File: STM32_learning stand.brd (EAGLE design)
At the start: 100 x 90 mm, 131 parts, among them J1 Power in, J10 RS-485_1, J11 RS-485_2, J12 FD CAN 1, J13 FD CAN 2, J15 Motor, J2 ST-link, J3 Encoder, J4 BMS_interface, J5 S6B-PH-K, J6 Current_1, J7 Current_2, J8 I2C, U1 TPS7A19, U10 THDV1450, U11 TCAN1042HGV, U12 DRV8701, U2 SGM2019, U3 STM32G431CBT, U4 REF3330, U5 REF3318, U6 ACS711KEXLT-15AB-T, U7 INA240A1, U8 24LC64T-I/SN, U9 CP2102N-A01-GQFN20, X1 CSTNE

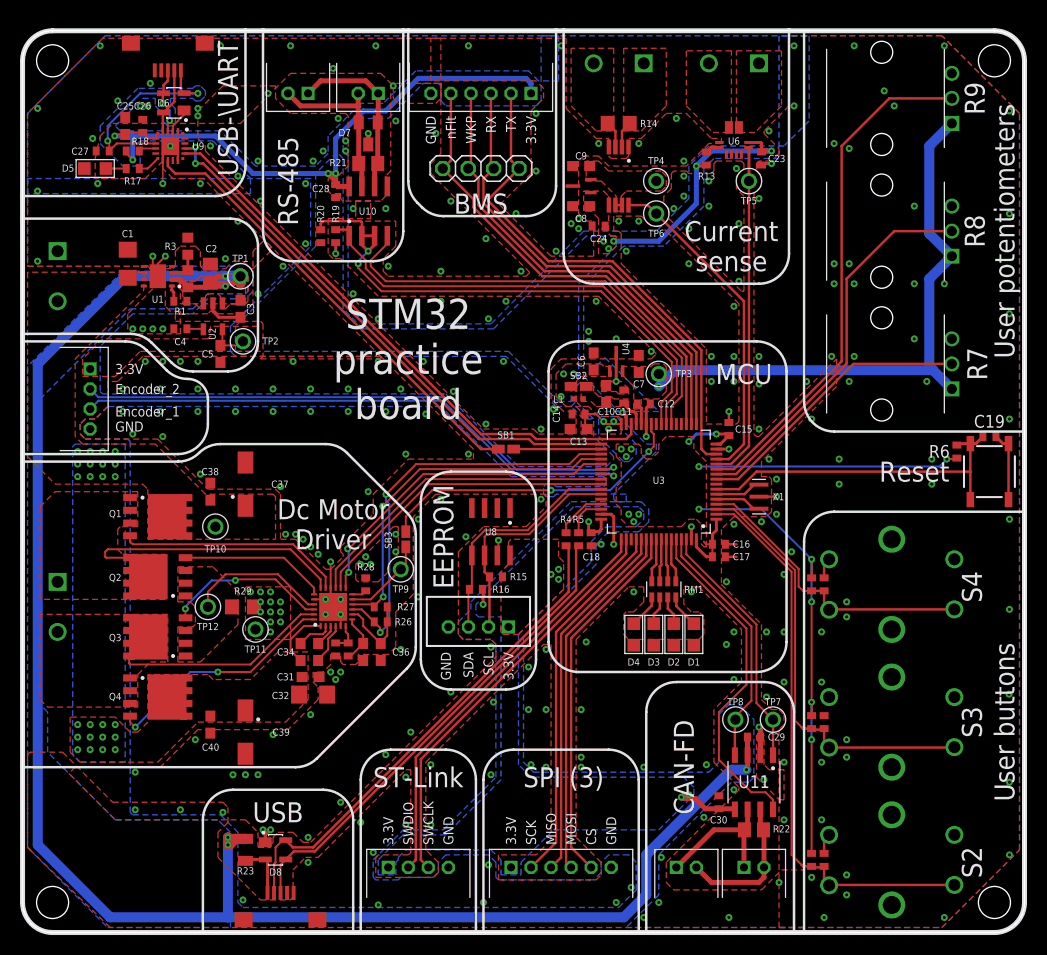
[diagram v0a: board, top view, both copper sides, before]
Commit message: small update
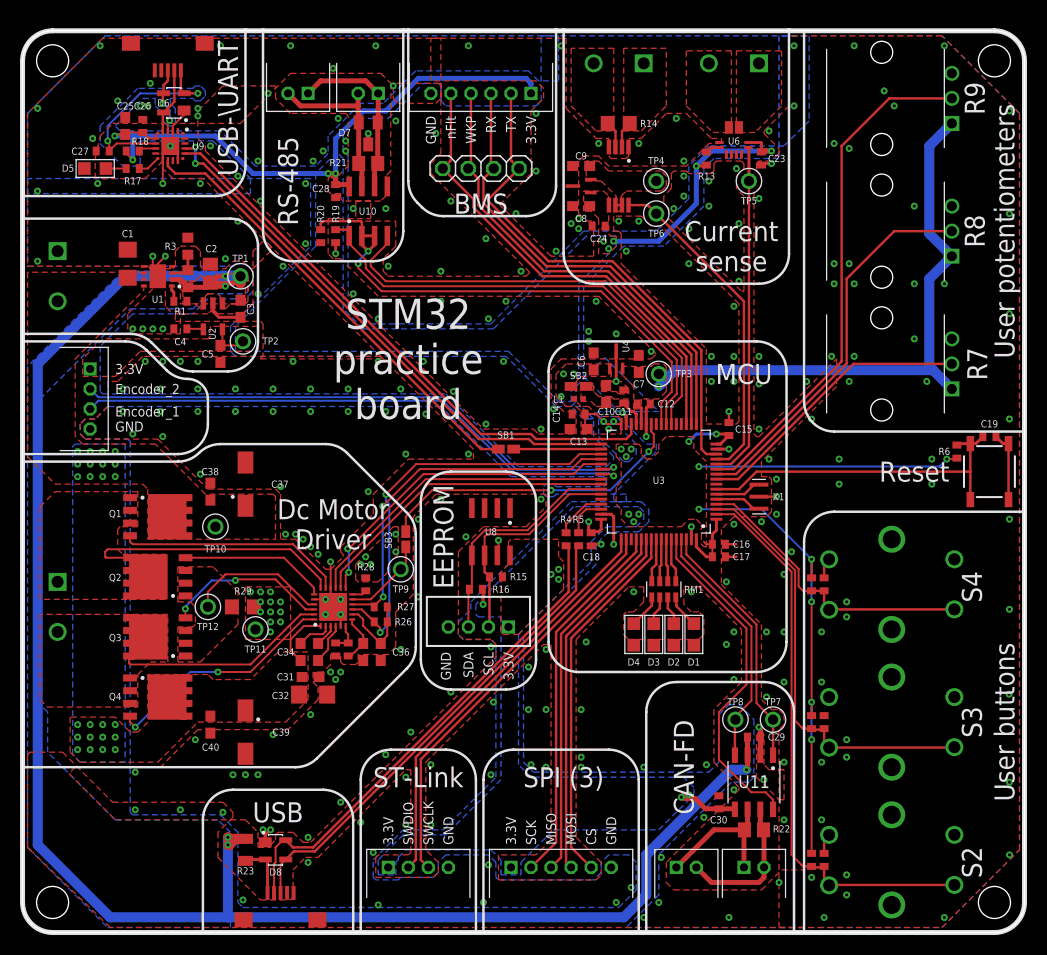
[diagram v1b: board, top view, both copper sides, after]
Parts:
- moved U4 0.25 mm to (59.2, 57.2)
